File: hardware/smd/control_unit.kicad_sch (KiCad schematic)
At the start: 32 parts, among them J3 UART, K1 SPST, 5V 72R, 10A 250VAC, Q1 NPN, 40V, 500mA, SW1 SW_Push, SW2 SW_Push, U5 ESP32-H2, Y1 32MHz ±10ppm CL8pF

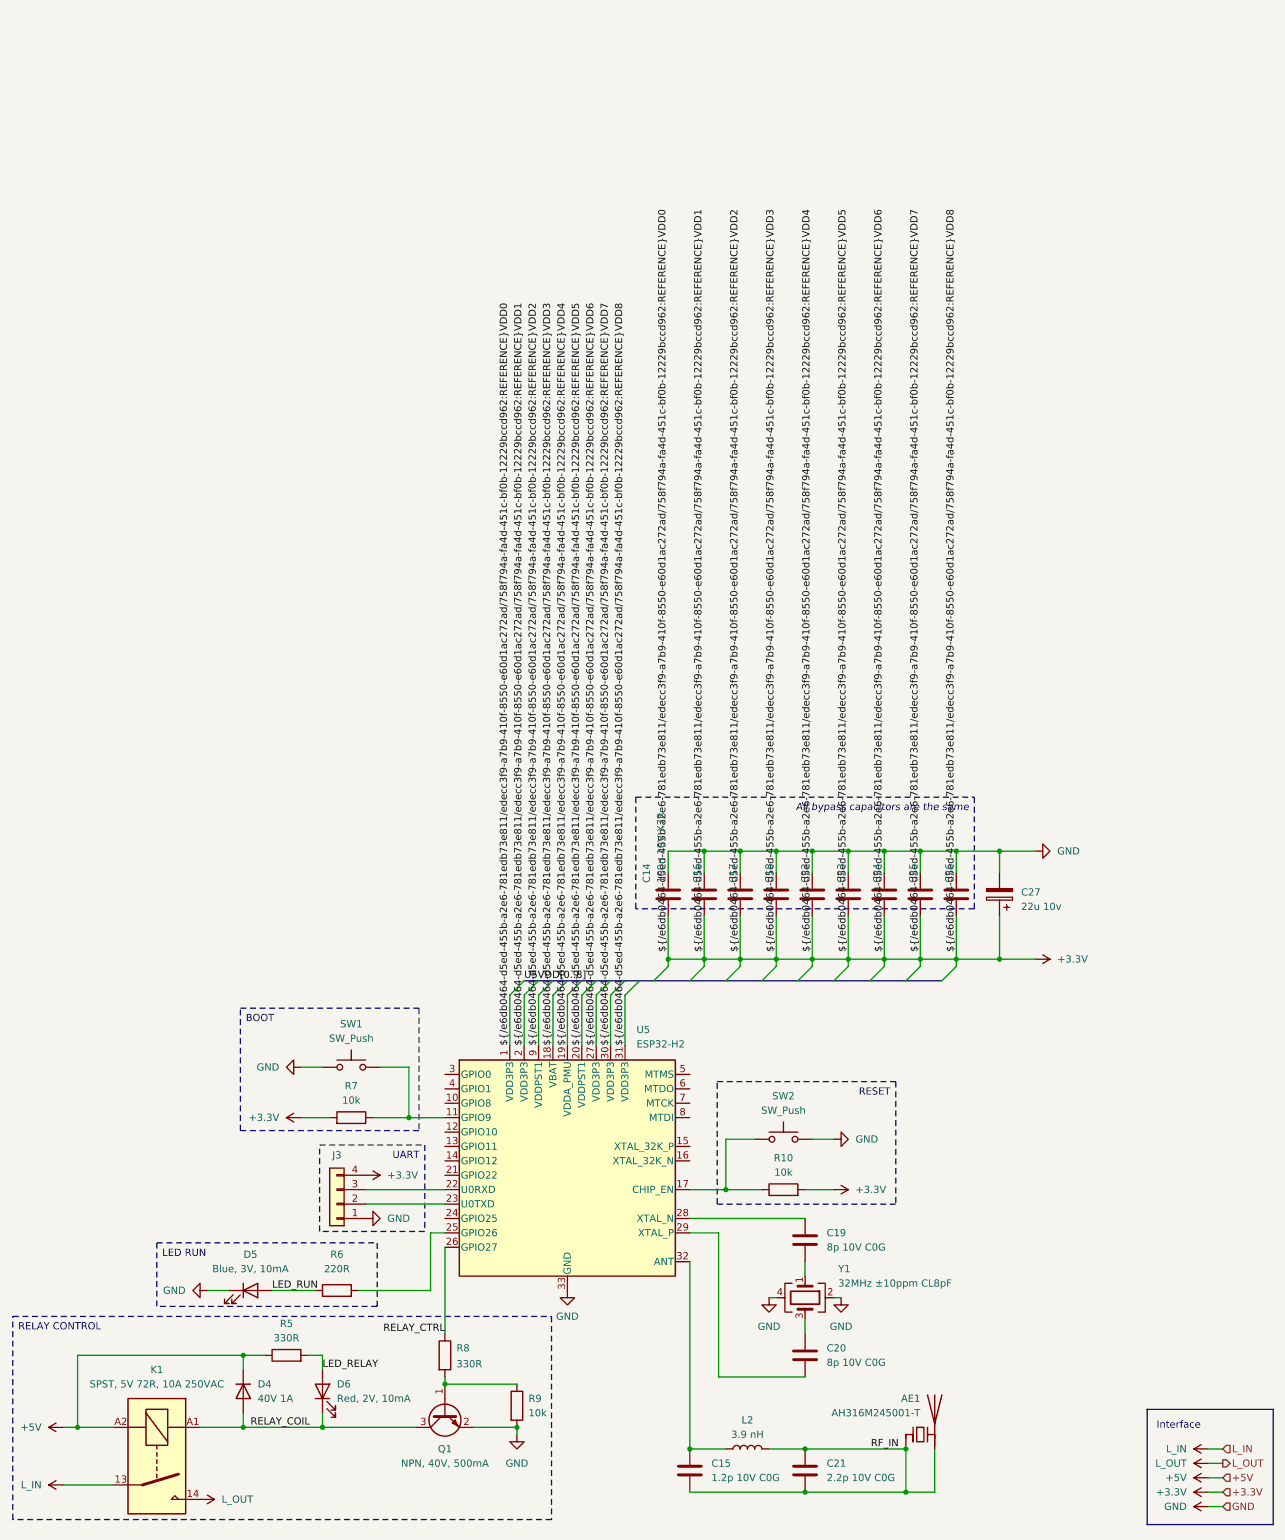
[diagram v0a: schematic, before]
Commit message: Complete PCB and schematics after fucking a lot of iterations
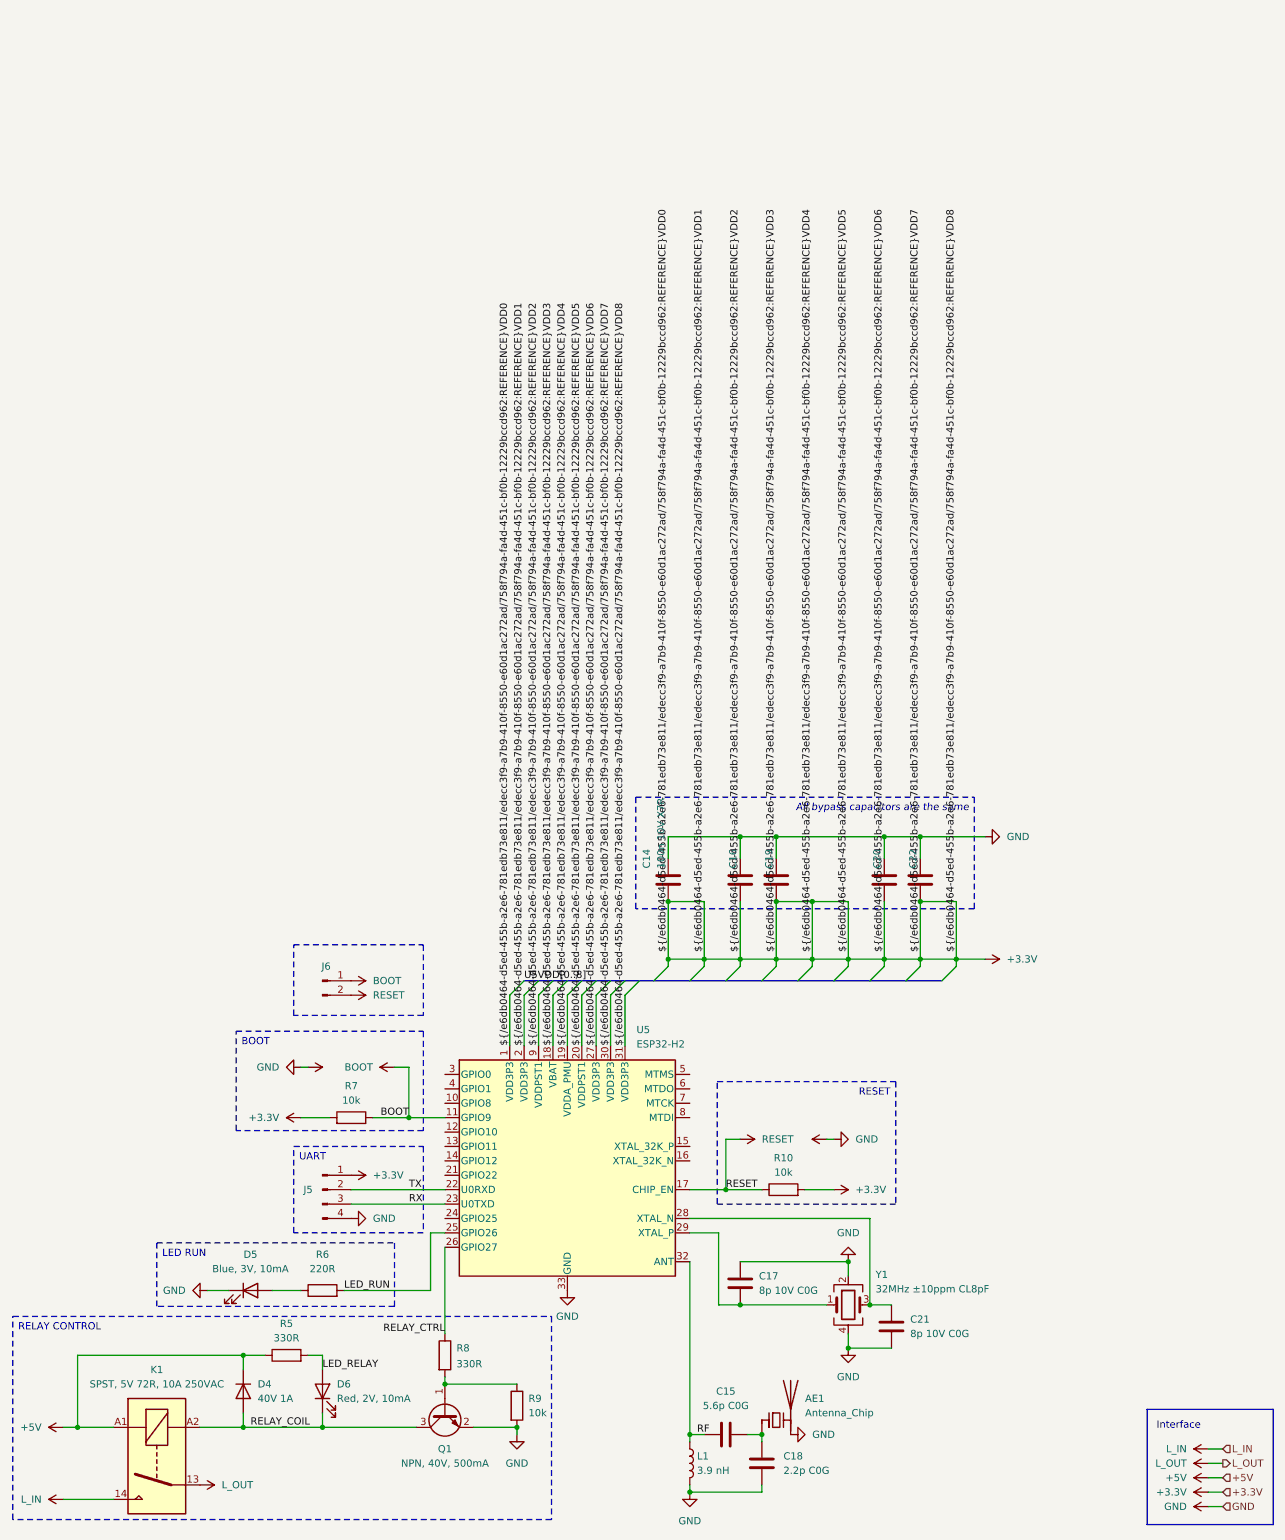
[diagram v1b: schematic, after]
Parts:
- removed C16, C22, C23, C26: 100n 10V X7R, Capacitor_SMD:C_0402_1005Metric, symbol Device:C
- removed C27: 22u 10v, Capacitor_SMD:CP_Elec_5x5.4, symbol Device:C_Polarized
- removed J3: UART, Connector_PinHeader_2.54mm:PinHeader_1x04_P2.54mm_Vertical, symbol Connector_Generic:Conn_01x04
- removed SW1, SW2: SW_Push, Button_Switch_SMD:SW_SPST_TL3305A, symbol Switch:SW_Push
- added J5: UART, Connector_PinHeader_1.27mm:PinHeader_1x04_P1.27mm_Vertical, symbol Connector:Conn_01x04_Pin
- added J6: Conn_01x02_Pin, Connector_PinHeader_1.27mm:PinHeader_1x02_P1.27mm_Vertical, symbol Connector:Conn_01x02_Pin
- AE1: value AH316M245001-T -> Antenna_Chip; footprint KiCadX_Antennas_SMD:AH316M245001_T -> KiCadX_Antennas_SMD:PCB_antenna_Espressif_2.4GHz_right; JLCPCB C3285031 -> (none); now left out of the parts list
- C15: value 1.2p 10V C0G -> 5.6p C0G; JLCPCB C285021 -> C85914
- C18: renamed from C21; value 2.2p 10V C0G -> 2.2p C0G
- K1: JLCPCB OJ-SH-105HM,000 -> C1564132
- renumbered C17 to C16, C20 to C17, C18 to C19, C24 to C20, C19 to C21, C25 to C22, L2 to L1
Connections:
- net +3.3V: now also J5.1 (Pin_1)
- net +5V: now also K1.A1; no longer K1.A2
- net GND: now also AE1.2 (PCB_Trace), C17.2, C18.1, C21.1, L1.2, J5.4 (Pin_4)
- net LED_RUN: now also R6.2, U5.25 (GPIO26); no longer D5.2 (A), R6.1
- net L_IN: now also K1.14; no longer K1.13
- net L_OUT: now also K1.13; no longer K1.14
- net RELAY_COIL: now also K1.A2; no longer K1.A1
- net at C17.1: now also U5.29 (XTAL_P), Y1.1; no longer Y1.3
- net RESET: now reaches R10.1, U5.17 (CHIP_EN)
- net RESET: now also J6.2 (Pin_2)
- net BOOT: now reaches R7.1, U5.11 (GPIO9)
- net BOOT: now also J6.1 (Pin_1)
- net at C21.2: now also U5.28 (XTAL_N), Y1.3; no longer Y1.1
- net TX: now reaches U5.22 (U0RXD)
- net TX: now also J5.2 (Pin_2)
- net RX: now reaches U5.23 (U0TXD)
- net RX: now also J5.3 (Pin_3)
- net RF: now reaches C15.2, L1.1, U5.32 (ANT)
- net RF_IN: no longer names the net of AE1.1 (FEED), C15.1, C18.2
- net RF_IN: no longer AE1.2 (PCB_Trace), C18.1, L1.2
- new net: D5.2 (A), R6.1
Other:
- moved on the sheet: C14, C15, C16, C17, C18, C19, C20, C21, C22, K1, L1, R6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
